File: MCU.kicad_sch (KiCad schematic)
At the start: 9 parts, among them Q1 AO3401A, U16 STM32G081CBUx, Y1 32.768kHz

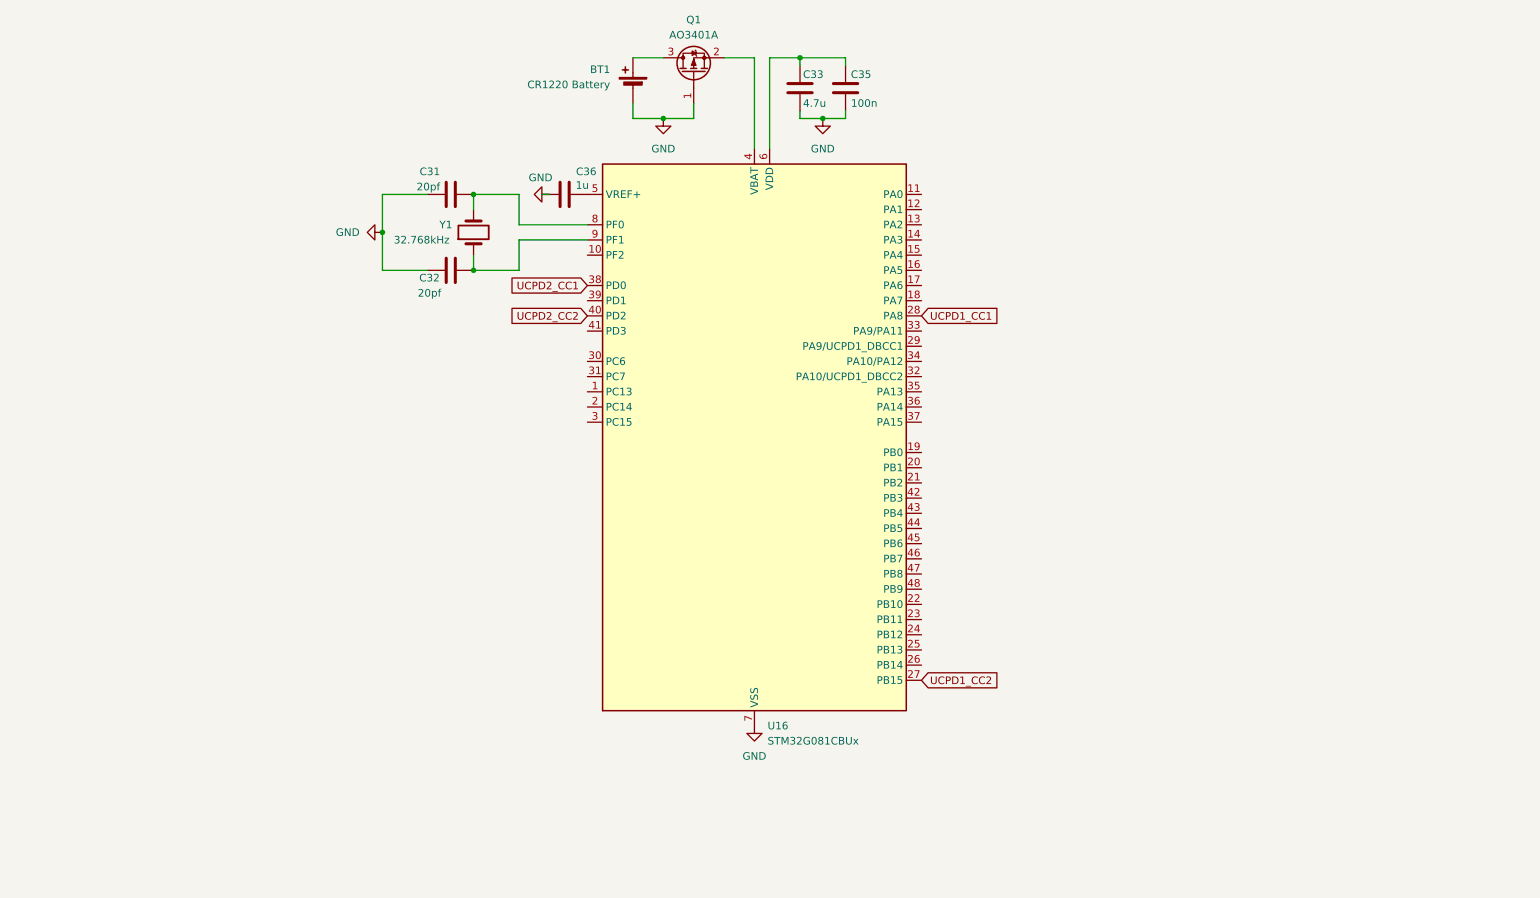
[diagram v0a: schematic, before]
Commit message: wip3
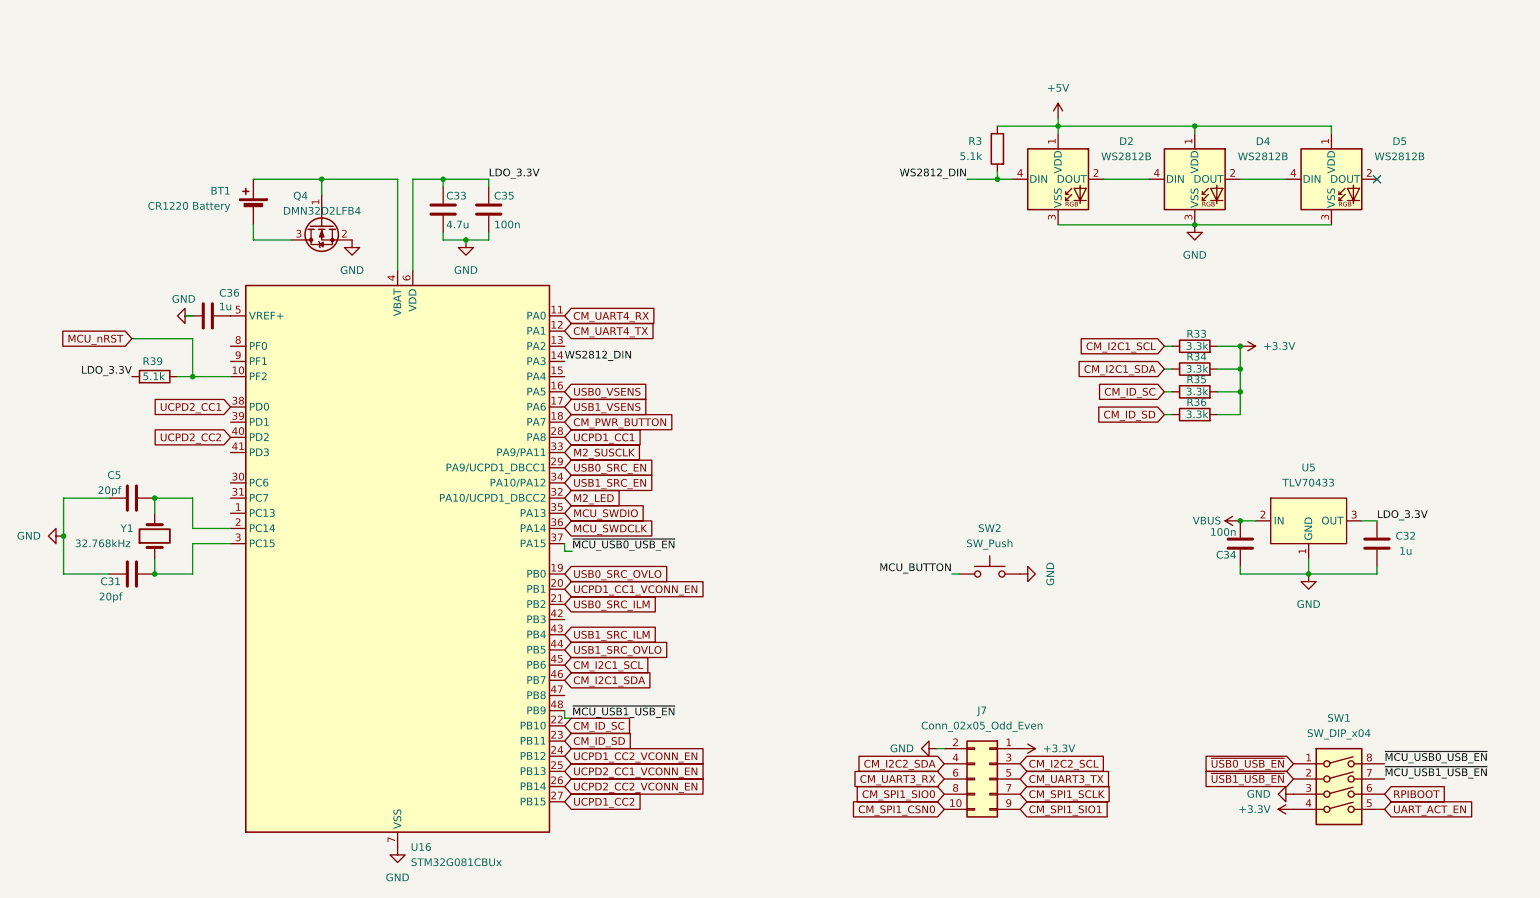
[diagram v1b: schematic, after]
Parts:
- removed Q1: AO3401A, Package_TO_SOT_SMD:SOT-23, symbol Device:Q_PMOS_GSD
- added C34: 100n, Capacitor_SMD:C_0402_1005Metric, symbol Device:C
- added C5: 20pf, Capacitor_SMD:C_0402_1005Metric, symbol Device:C
- added D2, D4, D5: WS2812B, PiCard:LED-SMD_4P-L4.0-W1.7-R, symbol LED:WS2812B
- added J7: Conn_02x05_Odd_Even, PiCard:HARWIN_M20-7810545R, symbol Connector_Generic:Conn_02x05_Odd_Even
- added Q4: DMN32D2LFB4, Package_DFN_QFN:Diodes_DFN1006-3, symbol Device:Q_NMOS_GSD
- added R3, R39: 5.1k, Resistor_SMD:R_0402_1005Metric, symbol Device:R
- added R33, R34, R35, R36: 3.3k, Resistor_SMD:R_0402_1005Metric, symbol Device:R
- added SW1: SW_DIP_x04, PiCard:SW-SMD_8P-L11.1-W6.2-P2.54-LS7.8, symbol Switch:SW_DIP_x04
- added SW2: SW_Push, PiCard:SW-SMD_GT-TC020B-H035-L05, symbol Switch:SW_Push
- added U5: TLV70433, Package_TO_SOT_SMD:SOT-23-5, symbol PiCard:TLV70433
- C32: value 20pf -> 1u; footprint Capacitor_SMD:C_0402_1005Metric -> Capacitor_SMD:C_0603_1608Metric; LCSC (none) -> C15849; MPN (none) -> CL10A105KB8NNNC; Manufacturer (none) -> Samsung
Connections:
- net GND: now also C32.2, C34.1, C5.1, D2.3 (VSS), D4.3 (VSS), D5.3 (VSS), J7.2 (Pin_2), Q4.2 (S), SW1.3, SW2.2, U5.1 (GND); no longer BT1.2 (-), C32.1
- net MCU_nRST: now reaches U16.10 (PF2)
- net MCU_nRST: now also R39.1
- net CM_UART4_RX: now reaches U16.11 (PA0)
- net CM_UART4_TX: now reaches U16.12 (PA1)
- net WS2812_DIN: now reaches U16.14 (PA3)
- net WS2812_DIN: now also D2.4 (DIN), R3.2
- net USB0_VSENS: now reaches U16.16 (PA5)
- net USB1_VSENS: now reaches U16.17 (PA6)
- net CM_PWR_BUTTON: now reaches U16.18 (PA7)
- net USB0_SRC_OVLO: now reaches U16.19 (PB0)
- net at U16.2 (PC14): now also Y1.2, C5.2
- net UCPD1_CC1_VCONN_EN: now reaches U16.20 (PB1)
- net USB0_SRC_ILM: now reaches U16.21 (PB2)
- net CM_ID_SC: now reaches U16.22 (PB10)
- net CM_ID_SC: now also R35.1
- net CM_ID_SD: now reaches U16.23 (PB11)
- net CM_ID_SD: now also R36.1
- net UCPD1_CC2_VCONN_EN: now reaches U16.24 (PB12)
- net UCPD2_CC1_VCONN_EN: now reaches U16.25 (PB13)
- net UCPD2_CC2_VCONN_EN: now reaches U16.26 (PB14)
- net USB0_SRC_EN: now reaches U16.29 (PA9/UCPD1_DBCC1)
- net at U16.3 (PC15): now also C31.2, Y1.1
- net M2_LED: now reaches U16.32 (PA10/UCPD1_DBCC2)
- net M2_SUSCLK: now reaches U16.33 (PA9/PA11)
- net USB1_SRC_EN: now reaches U16.34 (PA10/PA12)
- net MCU_SWDIO: now reaches U16.35 (PA13)
- net MCU_SWDCLK: now reaches U16.36 (PA14)
- net ~{MCU_USB0_USB_EN}: now reaches U16.37 (PA15)
- net ~{MCU_USB0_USB_EN}: now also SW1.8
- net at U16.4 (VBAT): now also BT1.1 (+), Q4.1 (G)
- net USB1_SRC_ILM: now reaches U16.43 (PB4)
- net USB1_SRC_OVLO: now reaches U16.44 (PB5)
- net CM_I2C1_SCL: now reaches U16.45 (PB6)
- net CM_I2C1_SCL: now also R33.1
- net CM_I2C1_SDA: now reaches U16.46 (PB7)
- net CM_I2C1_SDA: now also R34.1
- net ~{MCU_USB1_USB_EN}: now reaches U16.48 (PB9)
- net ~{MCU_USB1_USB_EN}: now also SW1.7
- net LDO_3.3V: now reaches C33.1, C35.2, U16.6 (VDD)
- net LDO_3.3V: now also C32.1, R39.2, U5.3 (OUT)
- new net: D4.2 (DOUT), D5.4 (DIN)
- new net: BT1.2 (-), Q4.3 (D)
- new net: D2.2 (DOUT), D4.4 (DIN)
- new net +3.3V: J7.1 (Pin_1), R33.2, R34.2, R35.2, R36.2, SW1.4
- new net +5V: D2.1 (VDD), D4.1 (VDD), D5.1 (VDD), R3.1
- new net CM_I2C2_SCL: J7.3 (Pin_3)
- new net CM_I2C2_SDA: J7.4 (Pin_4)
- new net CM_SPI1_CSN0: J7.10 (Pin_10)
- new net CM_SPI1_SCLK: J7.7 (Pin_7)
- new net CM_SPI1_SIO0: J7.8 (Pin_8)
- new net CM_SPI1_SIO1: J7.9 (Pin_9)
- new net CM_UART3_RX: J7.6 (Pin_6)
- new net CM_UART3_TX: J7.5 (Pin_5)
- new net MCU_BUTTON: SW2.1
- new net RPIBOOT: SW1.6
- new net UART_ACT_EN: SW1.5
- new net VBUS: C34.2, U5.2 (IN)
- new net ~{USB0_USB_EN}: SW1.1
- new net ~{USB1_USB_EN}: SW1.2
- now unconnected: U16.8 (PF0), U16.9 (PF1)
- no-connect marks 0 -> 1
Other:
- moved on the sheet: BT1, C33, C35, C36, U16
